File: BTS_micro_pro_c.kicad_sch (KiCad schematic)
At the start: 11 parts, among them J2 I2C, J3 Analog, J6 Analog, J7 Digital, P1 USB_C_Plug_USB2.0, U1 ATmega32U4-A, U3 AMS1117-3.3, Y1 Crystal

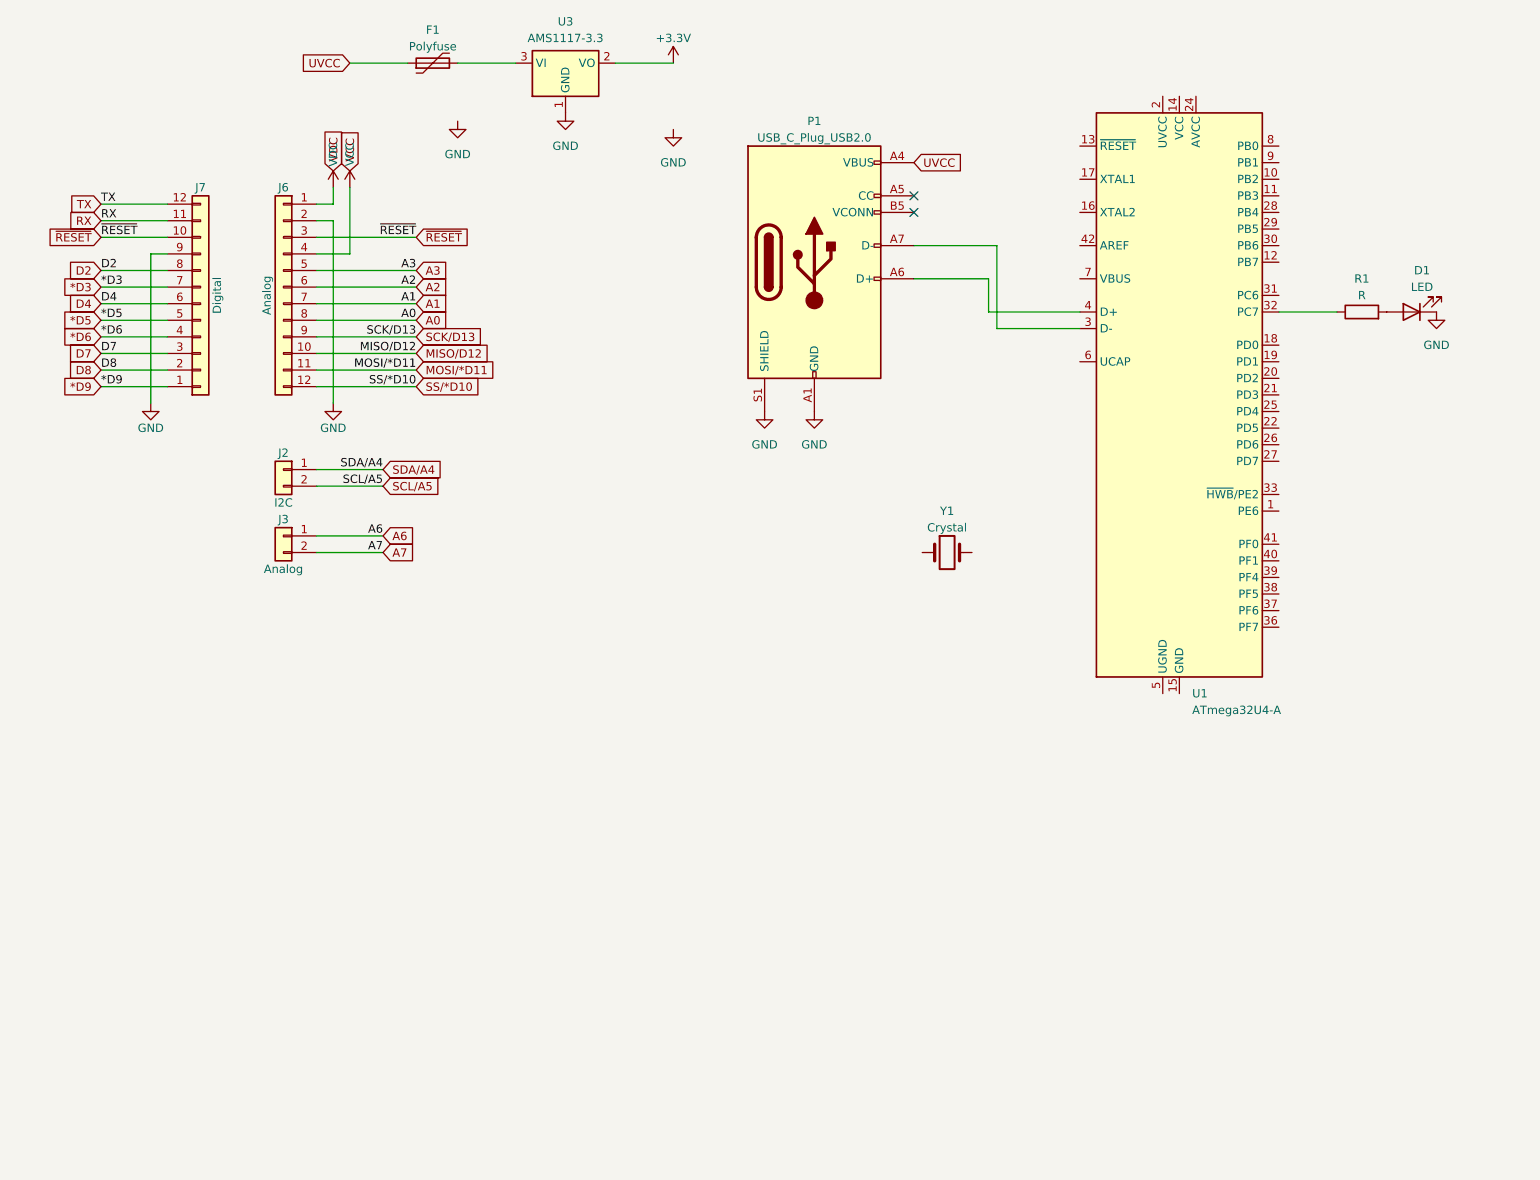
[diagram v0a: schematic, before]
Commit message: More progress.
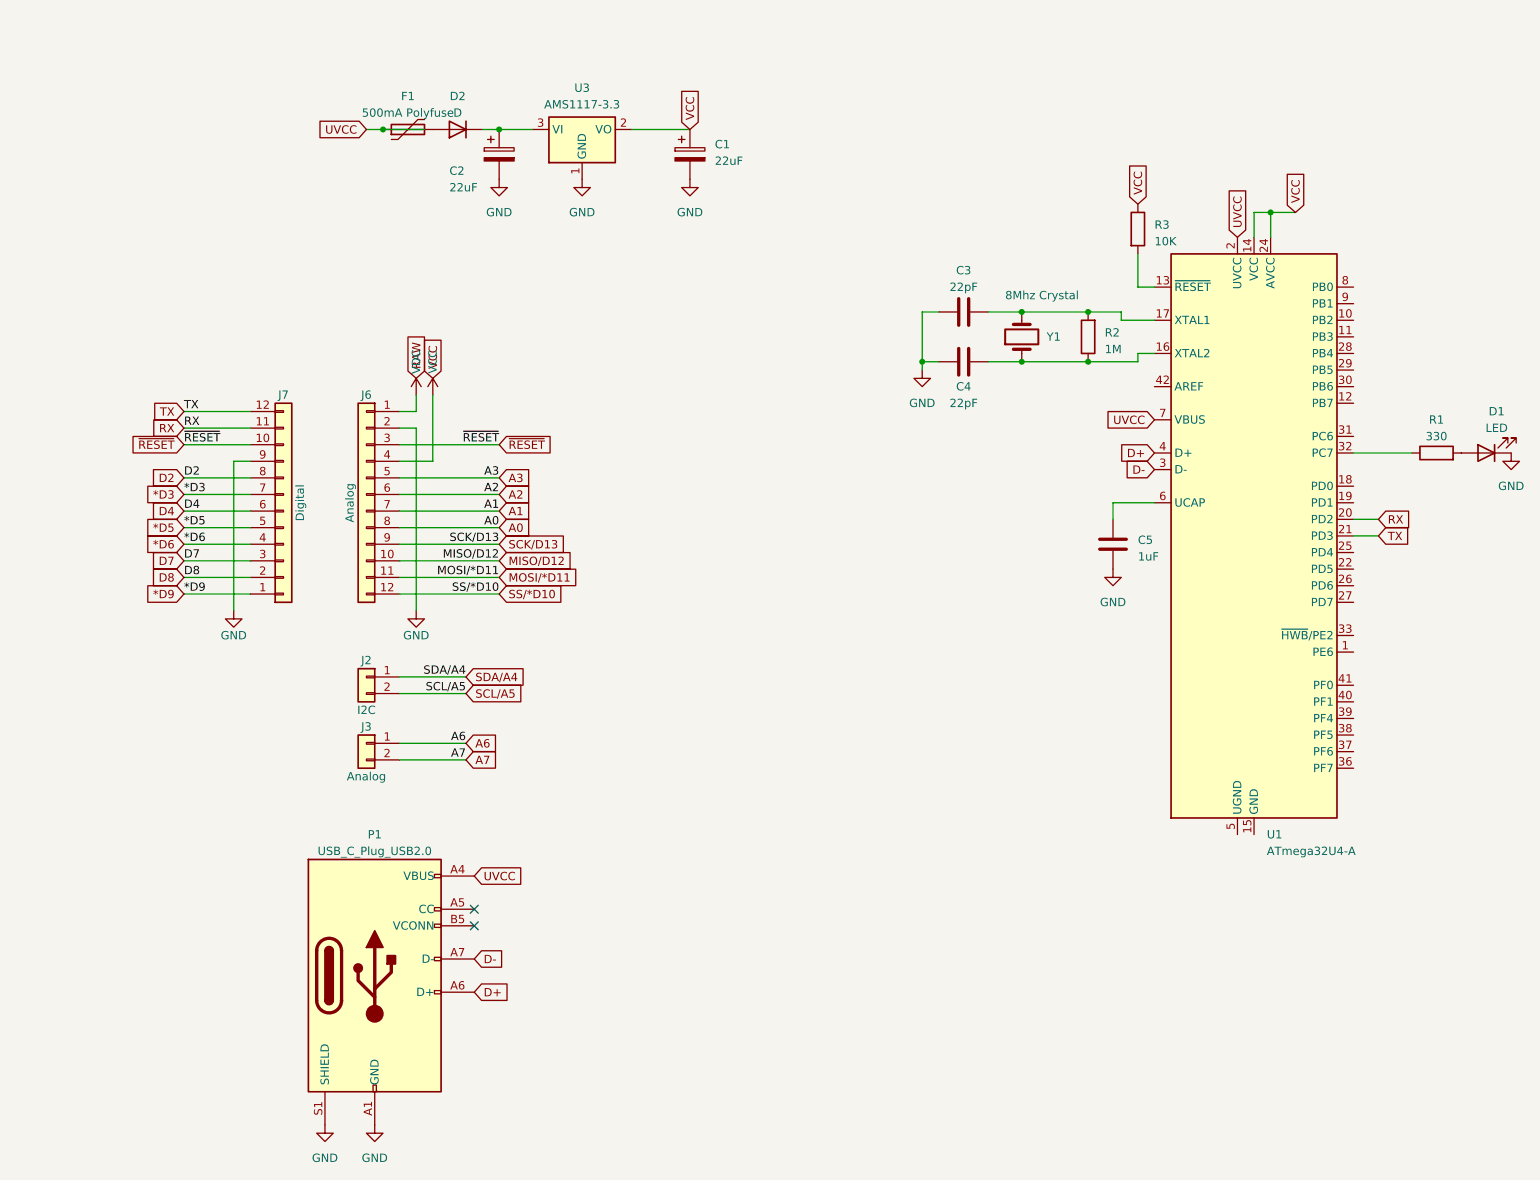
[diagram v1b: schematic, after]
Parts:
- added C1, C2: 22uF, symbol Device:C_Polarized
- added C3, C4: 22pF, symbol Device:C
- added C5: 1uF, symbol Device:C
- added D2: D, symbol Device:D
- added R2: 1M, symbol Device:R
- added R3: 10K, symbol Device:R
- F1: value Polyfuse -> 500mA Polyfuse
- R1: value R -> 330
- Y1: value Crystal -> 8Mhz Crystal
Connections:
- net +3.3V is gone; now on net VCC: U3.2 (VO)
- net GND: now also C1.2, C2.2, C3.1, C4.2, C5.2
- net RX: now also U1.20 (PD2)
- net TX: now also U1.21 (PD3)
- net UVCC: now also U1.2 (UVCC), U1.7 (VBUS)
- net VCC: now also U1.14 (VCC), U1.24 (AVCC), U1.34 (VCC), U1.44 (AVCC), C1.1, R3.1
- net at U3.3 (VI): now also C2.1, D2.1 (K); no longer F1.2
- net at Y1.1: now also U1.16 (XTAL2), C4.1, R2.1
- net at Y1.2: now also U1.17 (XTAL1), C3.2, R2.2
- net D+: now reaches P1.A6 (D+), U1.4 (D+)
- net D-: now reaches P1.A7 (D-), U1.3 (D-)
- net at U1.13 (~{RESET}): now also R3.2
- net at U1.6 (UCAP): now also C5.1
- new net: D2.2 (A), F1.2
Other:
- moved on the sheet: D1, F1, J2, J3, J6, J7, P1, R1, U1, U3, Y1
